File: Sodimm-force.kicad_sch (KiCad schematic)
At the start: 1 part, among them J1 SODIMM-200_Split

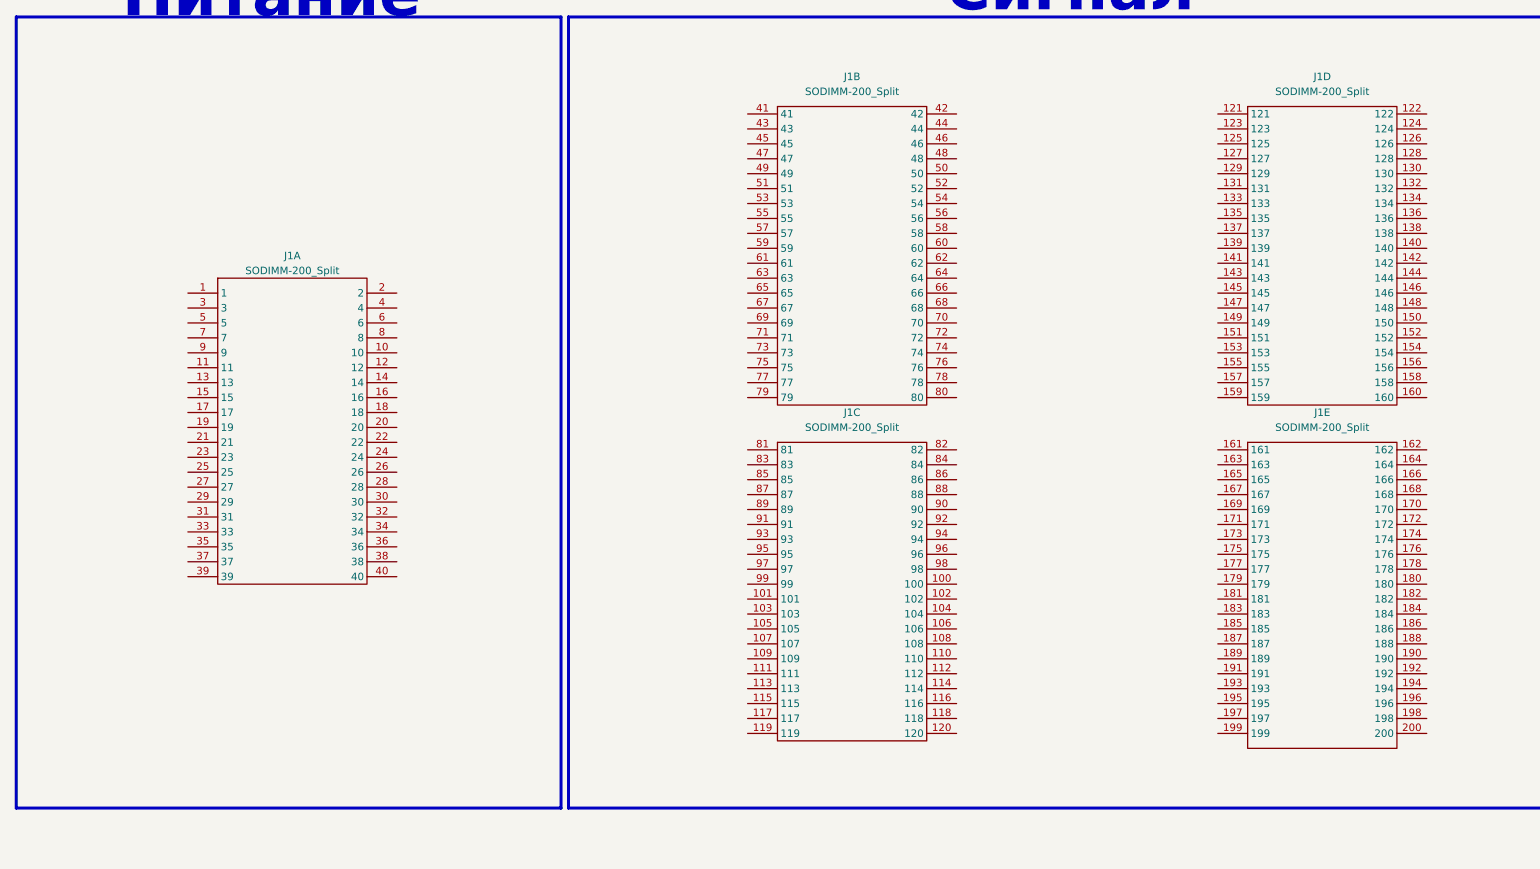
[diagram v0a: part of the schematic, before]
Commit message: Схема закончена, часть компонентов расставлена на плате
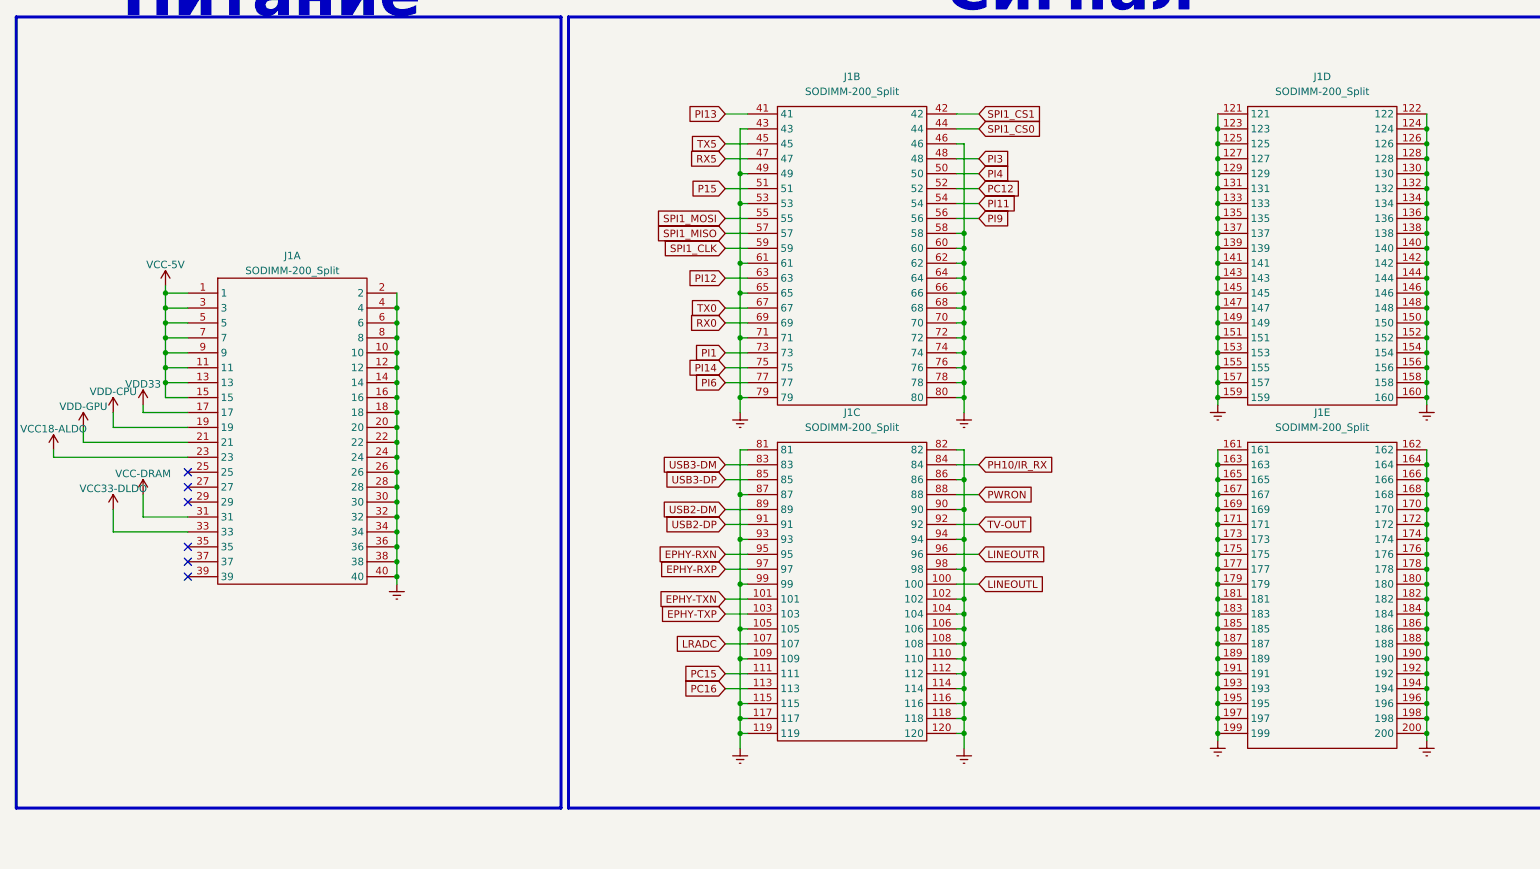
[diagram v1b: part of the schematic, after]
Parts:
- J1: footprint (none) -> Connector_PCBEdge:SODIMM-200_2.5V_Card_edge
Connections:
- net Earth: now reaches J1.121
- net Earth: now also J1.10, J1.102, J1.104, J1.105, J1.106, J1.108, J1.109, J1.110, J1.112, J1.114, J1.115, J1.116, J1.117, J1.118, J1.119, J1.12, J1.120, J1.122, J1.123, J1.124, J1.125, J1.126, J1.127, J1.128, J1.129, J1.130, J1.131, J1.132, J1.133, J1.134, J1.135, J1.136, J1.137, J1.138, J1.139, J1.14, J1.140, J1.141, J1.142, J1.143, J1.144, J1.145, J1.146, J1.147, J1.148, J1.149, J1.150, J1.151, J1.152, J1.153, J1.154, J1.155, J1.156, J1.157, J1.158, J1.159, J1.16, J1.160, J1.161, J1.162, J1.163, J1.164, J1.165, J1.166, J1.167, J1.168, J1.169, J1.170, J1.171, J1.172, J1.173, J1.174, J1.175, J1.176, J1.177, J1.178, J1.179, J1.18, J1.180, J1.181, J1.182, J1.183, J1.184, J1.185, J1.186, J1.187, J1.188, J1.189, J1.190, J1.191, J1.192, J1.193, J1.194, J1.195, J1.196, J1.197, J1.198, J1.199, J1.2, J1.20, J1.200, J1.22, J1.24, J1.26, J1.28, J1.30, J1.32, J1.34, J1.36, J1.38, J1.4, J1.40, J1.43, J1.46, J1.49, J1.53, J1.58, J1.6, J1.60, J1.61, J1.62, J1.64, J1.65, J1.66, J1.68, J1.70, J1.71, J1.72, J1.74, J1.76, J1.78, J1.79, J1.8, J1.80, J1.81, J1.82, J1.86, J1.87, J1.90, J1.93, J1.94, J1.98, J1.99
- net LINEOUTL: now reaches J1.100
- net EPHY-TXN: now reaches J1.101
- net EPHY-TXP: now reaches J1.103
- net LRADC: now reaches J1.107
- net PC15: now reaches J1.111
- net PC16: now reaches J1.113
- net USB3-DM: now reaches J1.83
- net PH10/IR_RX: now reaches J1.84
- net USB3-DP: now reaches J1.85
- net PWRON: now reaches J1.88
- net USB2-DM: now reaches J1.89
- net USB2-DP: now reaches J1.91
- net TV-OUT: now reaches J1.92
- net EPHY-RXN: now reaches J1.95
- net LINEOUTR: now reaches J1.96
- net EPHY-RXP: now reaches J1.97
- net VCC-5V: now reaches J1.1
- net VCC-5V: now also J1.11, J1.13, J1.15, J1.3, J1.5, J1.7, J1.9
- net VDD33: now reaches J1.17
- net VDD-CPU: now reaches J1.19
- net VDD-GPU: now reaches J1.21
- net VCC18-ALDO: now reaches J1.23
- net VCC-DRAM: now reaches J1.31
- net VCC33-DLDO: now reaches J1.33
- net PI13: now reaches J1.41
- net SPI1_CS1: now reaches J1.42
- net SPI1_CS0: now reaches J1.44
- net TX5: now reaches J1.45
- net RX5: now reaches J1.47
- net PI3: now reaches J1.48
- net PI4: now reaches J1.50
- net P15: now reaches J1.51
- net PC12: now reaches J1.52
- net PI11: now reaches J1.54
- net SPI1_MOSI: now reaches J1.55
- net PI9: now reaches J1.56
- net SPI1_MISO: now reaches J1.57
- net SPI1_CLK: now reaches J1.59
- net PI12: now reaches J1.63
- net TX0: now reaches J1.67
- net RX0: now reaches J1.69
- net PI1: now reaches J1.73
- net PI14: now reaches J1.75
- net PI6: now reaches J1.77
- no-connect marks 0 -> 6
